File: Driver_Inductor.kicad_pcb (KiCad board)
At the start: 6 copper layers, 120.5 x 72.9 mm, 99 parts, among them J1 2-338069-0, J2 DC+, J3 DC-, J4 OUT1, J5 OUT2, U1 R-783.3-1.0, U2 R-785.0-1.0, U3 LM1117GS-3.3, U4 LMV331, U5 ADuM1200AR, U6 74LVC1G04

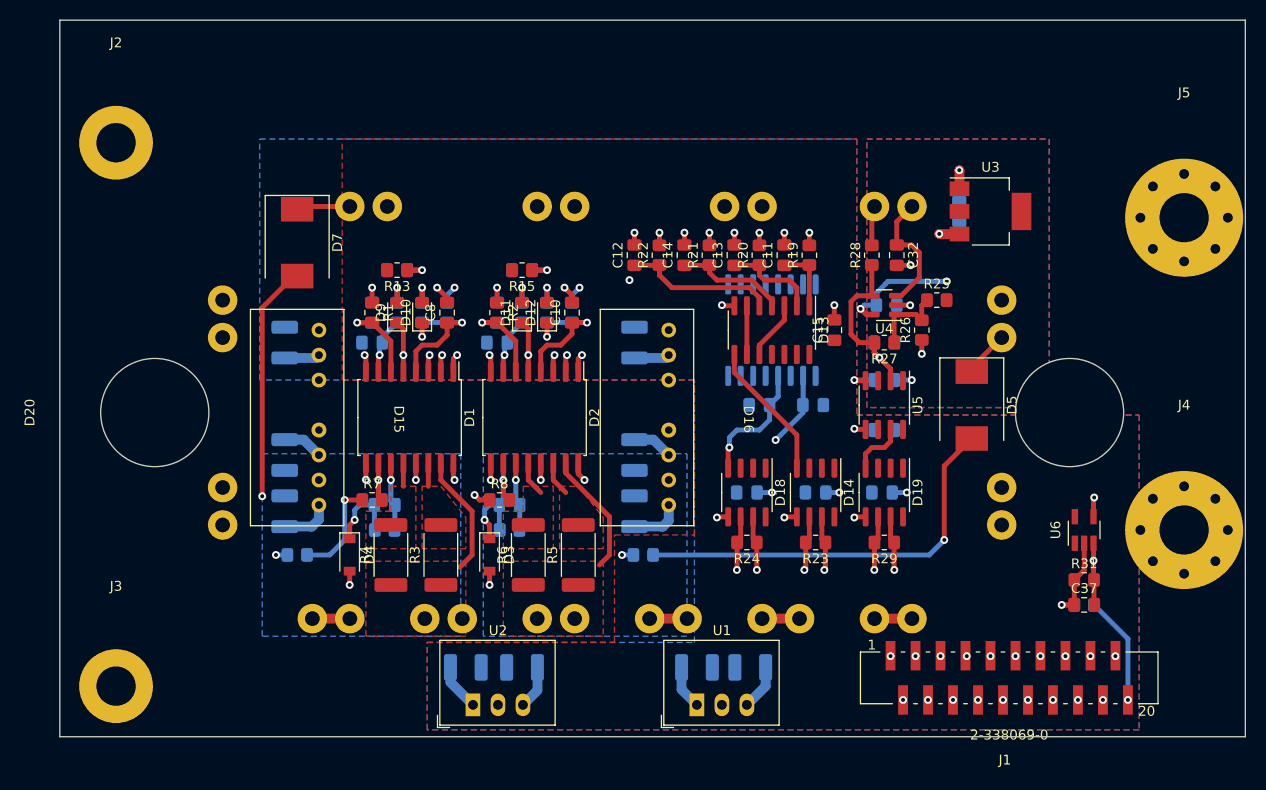
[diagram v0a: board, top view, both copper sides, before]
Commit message: Тестовая версия
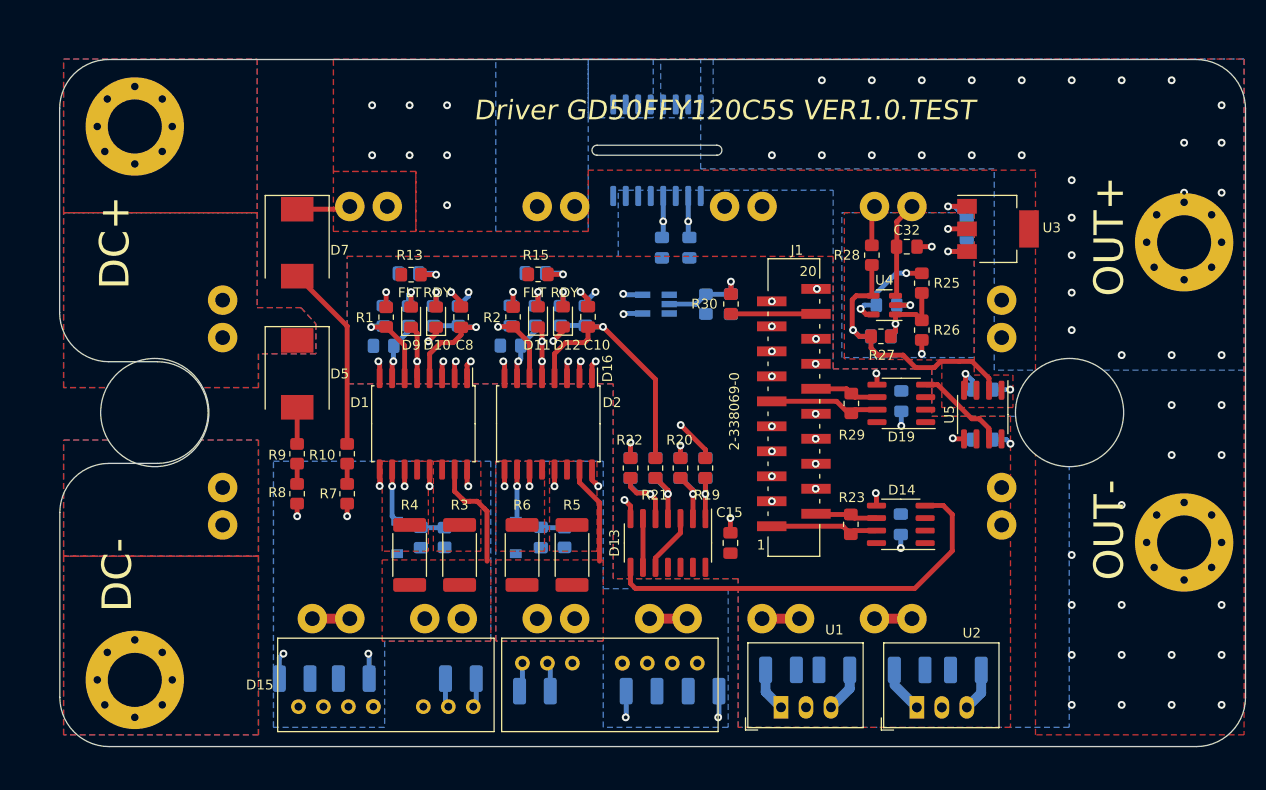
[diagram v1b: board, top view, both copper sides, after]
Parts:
- removed C29: 2.2u, Capacitor_SMD:C_0805_2012Metric_Pad1.18x1.45mm_HandSolder
- removed D18: ADM3485E, Package_SO:SOIC-8_3.9x4.9mm_P1.27mm
- removed R24: 120, Resistor_SMD:R_0805_2012Metric_Pad1.20x1.40mm_HandSolder
- C11, C12, C13, C14, C37, D3, D4, R31, U6: moved to B.Cu
- J2, J3: footprint Connector Power:M4 -> Connector_Power:M5
- J4, J5: footprint Connector Power:M5 -> Connector_Power:M5
- R10, R30, R9: moved to F.Cu
- moved D5 68.7 mm to (113.0, 93.3)
- moved U6 49.2 mm to (149.5, 86.3), turned to 180 degrees
- moved R31 47.6 mm to (154.6, 86.3), turned to -90 degrees
- moved R30 47.2 mm to (157.1, 86.2), turned to -90 degrees
- moved C37 47.2 mm to (157.1, 86.3), turned to -90 degrees
- moved C22 45.1 mm to (181.0, 123.4)
- moved U2 45.1 mm to (176.0, 127.3)
- moved C20 45.1 mm to (175.3, 123.4)
- moved C18 38.6 mm to (129.7, 124.3), turned to 0 degrees
- moved C17 36.9 mm to (137.2, 125.6), turned to 180 degrees
- moved R9 36.7 mm to (113.0, 101.5), turned to -90 degrees
- moved D15 30.0 mm to (121.9, 127.2), turned to 180 degrees
- moved D16 25.5 mm to (145.0, 122.8), turned to 0 degrees
- moved C15 24.1 mm to (157.1, 110.5)
- moved D13 24.1 mm to (150.7, 110.5)
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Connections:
- C25 pad 2: E1 -> E3
- C26 pad 1: E1 -> E3
- C28 pad 1: Net-(C28-Pad1) -> Current
- C30 pad 1: E1 -> E3
- D16 pad 7: E1 -> E3
- D17 pad 1: E3 -> OUT2
- D17 pad 12: Net-(C28-Pad1) -> Current
- D17 pad 2: E3 -> OUT2
- D17 pad 3: E3 -> OUT2
- D17 pad 4: E3 -> OUT2
- D17 pad 5: OUT+ -> OUT2_Sens
- D17 pad 6: OUT+ -> OUT2_Sens
- D17 pad 7: OUT+ -> OUT2_Sens
- D17 pad 8: OUT+ -> OUT2_Sens
- D20 pad 15: DESAT_H -> unconnected-(D20-Pad15)
- D20 pad 21: E3 -> OUT2
- D20 pad 22: E3 -> OUT2
- D20 pad 23: E1 -> OUT1
- D20 pad 24: E1 -> OUT1
- D20 pad 25: Net-(D20-Pad25) -> DESAT_H
- D20 pad 26: Net-(D20-Pad25) -> DESAT_H
- D7 pad 1: E1 -> OUT1
- J1 pad 1: GND -> Fault_N
- J1 pad 10: Fault_N -> +15V
- J1 pad 11: Temp_P -> Temp_N
- J1 pad 12: Temp_N -> Temp_P
- J1 pad 13: PWM2_P -> PWM1_P
- J1 pad 14: PWM2_N -> PWM1_N
- J1 pad 15: PWM1_P -> PWM2_P
- J1 pad 16: PWM1_N -> PWM2_N
- J1 pad 18: +15V -> Reset
- J1 pad 2: +15V -> Fault_P
- J1 pad 20: Reset -> Current
- J1 pad 7: Current_P -> GND
- J1 pad 8: Current_N -> +15V
- J1 pad 9: Fault_P -> GND
- J2 pad 1: Net-(D20-Pad25) -> DESAT_H
- J4 pad 1: E1 -> OUT1
- J5 pad 1: E3 -> OUT2_Sens
- U3 pad 3: E1 -> E3
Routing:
- net RST_H1: track 103.4 -> 33.5 mm
- net E3: track 8.36 -> 70.5 mm
- net PWM1_N: track 78.6 -> 28.7 mm
- net PWM1_P: track 71.4 -> 22.9 mm
- net PWM2_N: track 87.4 -> 42.1 mm
- net PWM2_P: track 80.5 -> 36.2 mm
- net Net-(D5-Pad2): track 41.7 -> 3.73 mm, vias 1 -> 0
- net Current_N: track 37.2 -> 0.00 mm, vias 2 -> 0
- net Current_P: track 33.5 -> 0.00 mm, vias 2 -> 0
- net -15V_H1: track 51.3 -> 20.1 mm, vias 7 -> 8
- net Net-(D13-Pad8): track 14.2 -> 43.0 mm
- net Net-(C5-Pad1): track 14.1 -> 37.9 mm
- net Current: track 0.00 -> 22.8 mm, vias 0 -> 2
- net Fault_P: track 28.2 -> 6.33 mm, vias 2 -> 0
- net Fault_N: track 31.9 -> 11.1 mm, vias 2 -> 0
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- added copper zone on In1.Cu, net +15V
- added copper zone on In3.Cu, net +15V_H1
- added copper zone on In3.Cu, net +15V_L1
- added copper zone on In3.Cu, net +3.3VA
- added copper zone on In3.Cu, net +3V3
- added copper zone on In4.Cu, net -15V_H1
- added copper zone on In4.Cu, net -15V_L1
- added copper zone on B.Cu, net DESAT_H
- added copper zone on F.Cu, net DESAT_H
- added copper zone on B.Cu, net E3
- added copper zone on In2.Cu, net GND
- added copper zone on B.Cu, net Net-(D20-Pad27)
- added copper zone on F.Cu, net Net-(D20-Pad27)
- added copper zone on B.Cu, net OUT1
- added copper zone on F.Cu, net OUT1
- added copper zone on In1.Cu, net OUT1
- added copper zone on In2.Cu, net OUT1
- added copper zone on B.Cu, net OUT2
- added copper zone on In3.Cu, net OUT2
- added copper zone on In4.Cu, net OUT2
- added copper zone on B.Cu, net OUT2_Sens
- added copper zone on In3.Cu, net OUT2_Sens
- added copper zone on In4.Cu, net OUT2_Sens
- removed copper zone on In2.Cu, net +15V
- removed copper zone on In1.Cu, net +15V_H1
- removed copper zone on In1.Cu, net +15V_L1
- removed copper zone on B.Cu, net -15V_H1
- removed copper zone on In2.Cu, net -15V_H1
- removed copper zone on In2.Cu, net -15V_L1
- removed copper zone on In1.Cu, net DESAT_H
- removed copper zone on In2.Cu, net DESAT_H
- removed copper zone on B.Cu, net E1
- removed copper zone on In3.Cu, net E1
- removed copper zone on In1.Cu, net E2
- removed copper zone on In4.Cu, net E3
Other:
- board size 120.5 x 72.9 mm -> 120.6 x 69.9 mm
- board text added: "DC+"
- board text added: "DC-"
- board text added: "Driver GD50FFY120C5S VER1.0.TEST"
- board text added: "FLT"
- board text added: "OUT+"
- board text added: "OUT-"
- board text added: "RDY"
